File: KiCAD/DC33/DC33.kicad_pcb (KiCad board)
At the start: 4 copper layers, 198.5 x 104.3 mm, 200 parts, among them J1 SAO, J2 PPTC201LFBN-RC, J3 PPTC201LFBN-RC, J4 282834-3, J5 282834-3, J6 FPC-30, J7 S2B-PH-K-S(LF)(SN), Q1 FDN359BN, Q2 CSD17576Q5B, Q3 CSD17576Q5B, U1 PICO2, U10 PCA9536DRG4, U11 ADG849YKSZ-REEL, U12 ADG849YKSZ-REEL, U13 MCP2558FD-H_SN, U14 ADG849YKSZ-REEL, U15 ADG849YKSZ-REEL, U16 ADG849YKSZ-REEL, U17 ADG849YKSZ-REEL, U18 ADG849YKSZ-REEL, U19 ADG849YKSZ-REEL, U2 TS5A3359DCUR, U20 MAX33046EASA+T, U21 ALM2403QPWPRQ1, U22 TMUX1108PWR, U23 TL431AIDBZR, U24 TMUX1108PWR, U25 TL431AIDBZR, U26 TL431AIDBZR, U27 TPS22810TDBVRQ1, U28 TL431AIDBZR, U29 TCAL9539PWR, U3 TPSM828303ARDSR, U30 TPS22810TDBVRQ1, U31 MCP2518FD, U4 ADR510ARTZ-REEL7, U5 MC3479, U6 LM4040D20IDBZR, U7 ISL21010CFH315Z-T7A, U8 BQ297xy, U9 BQ25895RTW, Y1 20MHz 18pF

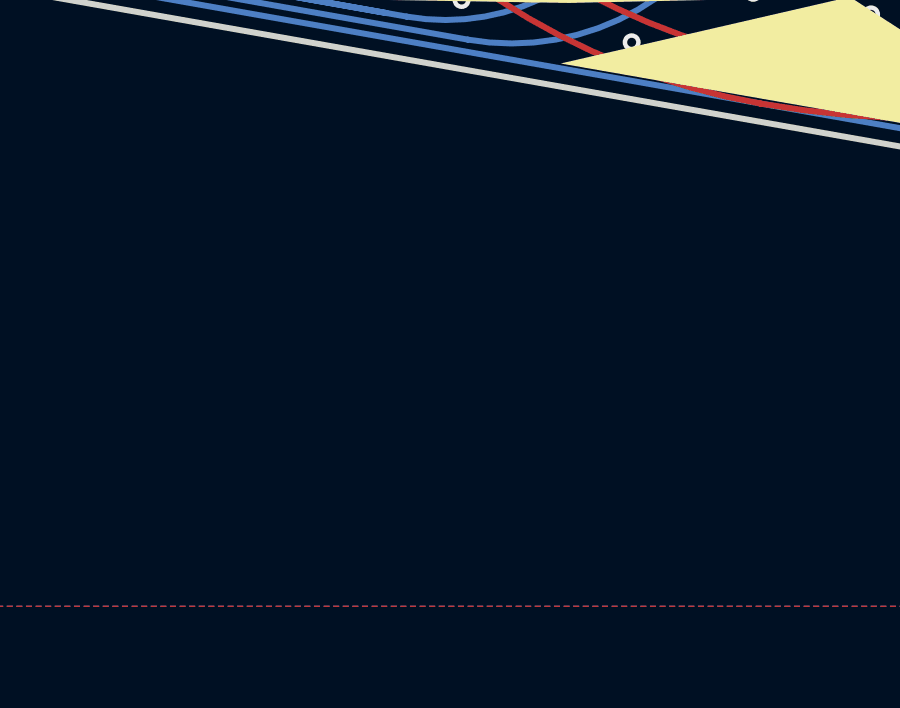
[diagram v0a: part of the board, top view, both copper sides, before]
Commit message: render
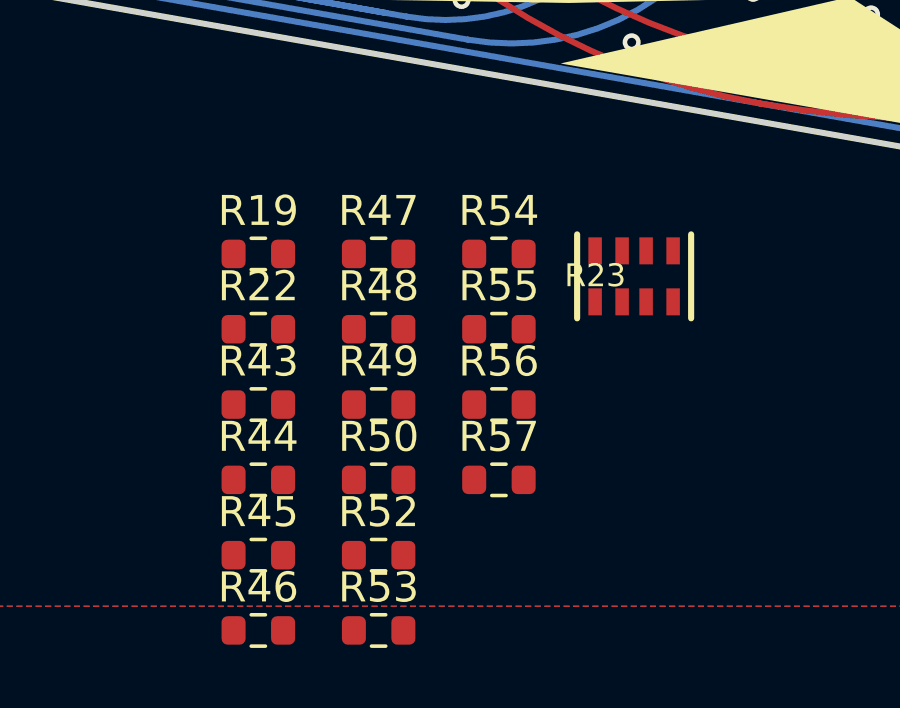
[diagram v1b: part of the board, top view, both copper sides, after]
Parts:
- added R19: 2k, Resistor_SMD:R_0603_1608Metric, F.Cu at (132.2, 151.3)
- added R22: 2k, Resistor_SMD:R_0603_1608Metric, F.Cu at (132.2, 153.9)
- added R23: 10k, Library:RESPACK_4X0603, F.Cu at (144.7, 152.1)
- added R43: 2k, Resistor_SMD:R_0603_1608Metric, F.Cu at (132.2, 156.4)
- added R44: 1k, Resistor_SMD:R_0603_1608Metric, F.Cu at (132.2, 158.9)
- added R45: 2k, Resistor_SMD:R_0603_1608Metric, F.Cu at (132.2, 161.4)
- added R46: 1k, Resistor_SMD:R_0603_1608Metric, F.Cu at (132.2, 163.9)
- added R47: 2k, Resistor_SMD:R_0603_1608Metric, F.Cu at (136.2, 151.3)
- added R48: 2k, Resistor_SMD:R_0603_1608Metric, F.Cu at (136.2, 153.9)
- added R49: 1k, Resistor_SMD:R_0603_1608Metric, F.Cu at (136.2, 156.4)
- added R50: 2k, Resistor_SMD:R_0603_1608Metric, F.Cu at (136.2, 158.9)
- added R52: 1k, Resistor_SMD:R_0603_1608Metric, F.Cu at (136.2, 161.4)
- added R53: 2k, Resistor_SMD:R_0603_1608Metric, F.Cu at (136.2, 163.9)
- added R54: 2.2k, Resistor_SMD:R_0603_1608Metric, F.Cu at (140.2, 151.3)
- added R55: 2.2k, Resistor_SMD:R_0603_1608Metric, F.Cu at (140.2, 153.9)
- added R56: 1k, Resistor_SMD:R_0603_1608Metric, F.Cu at (140.2, 156.4)
- added R57: 1k, Resistor_SMD:R_0603_1608Metric, F.Cu at (140.2, 158.9)
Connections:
- C25 pad 1: Net-(C25-Pad1) -> Net-(SW1-C)
- J7 pad 1: Net-(C25-Pad1) -> Net-(SW1-B)
- R18 pad 2: GND -> (no net)
- R18 pad 3: GND -> (no net)
- R18 pad 4: GND -> (no net)
- R18 pad 5: /Diff injector/H_V0 -> (no net)
- R18 pad 6: /Diff injector/H_V1 -> (no net)
- R18 pad 7: /Diff injector/H_V2 -> (no net)
- R31 pad 2: Net-(C25-Pad1) -> Net-(SW1-C)
- U9 pad 13: Net-(C25-Pad1) -> Net-(SW1-C)
- U9 pad 14: Net-(C25-Pad1) -> Net-(SW1-C)
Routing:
- net Net-(C25-Pad1): track 25.1 -> 0.00 mm
- net (no net): track 0.00 -> 25.1 mm
